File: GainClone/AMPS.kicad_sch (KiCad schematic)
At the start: 26 parts, among them U1 LM3886, U3 LM3886

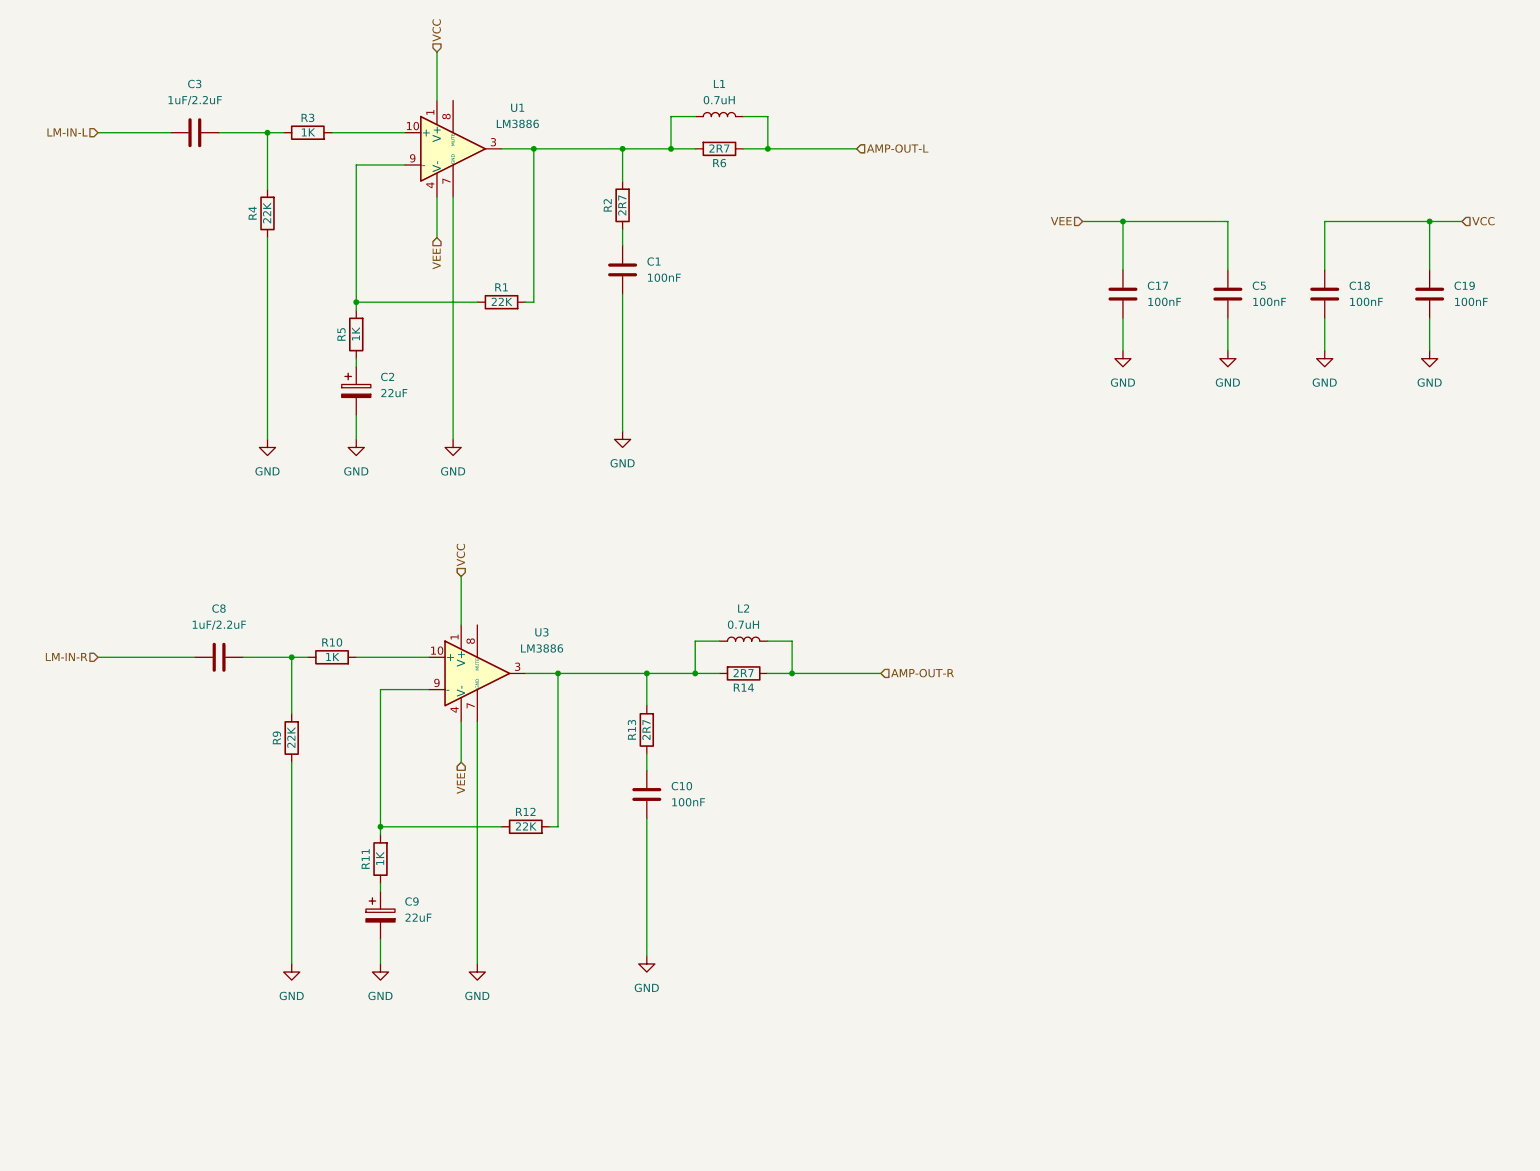
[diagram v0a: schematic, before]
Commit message: commit
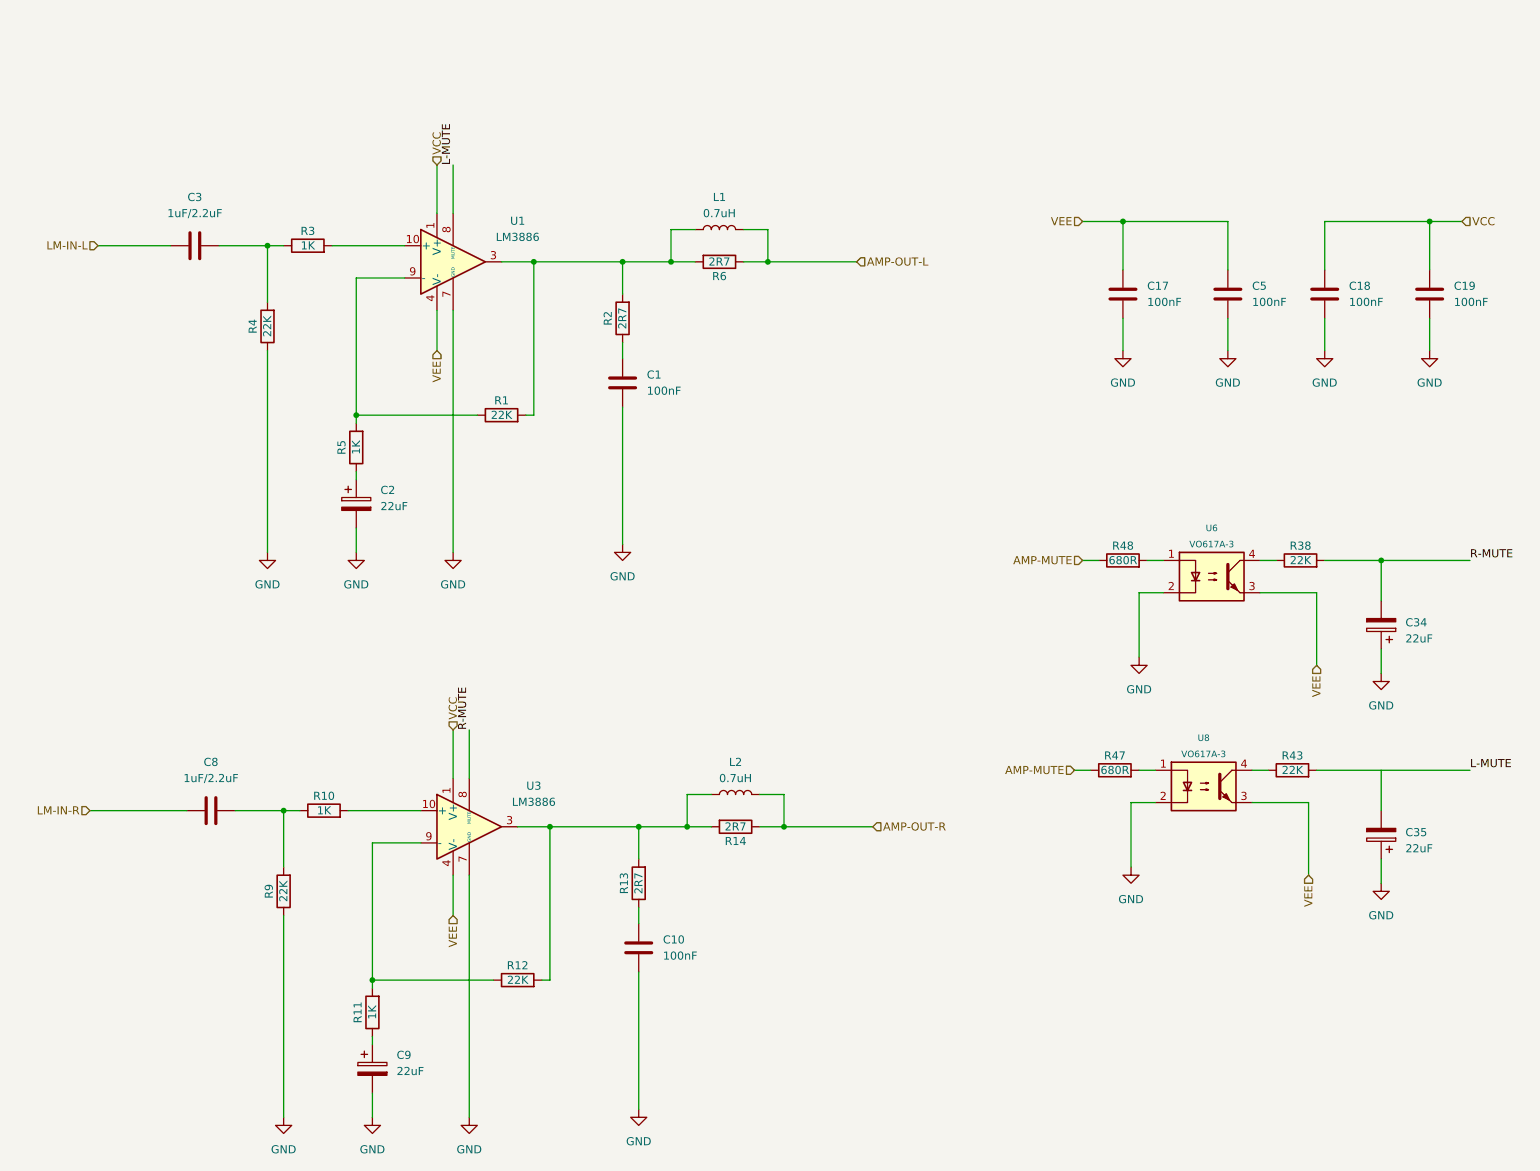
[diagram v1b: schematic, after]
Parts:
- added C34, C35: 22uF, Capacitor_THT:CP_Radial_D5.0mm_P2.50mm, symbol Device:C_Polarized
- added R38, R43: 22K, Resistor_SMD:R_0805_2012Metric_Pad1.20x1.40mm_HandSolder, symbol Device:R
- added R47, R48: 680R, Resistor_SMD:R_0805_2012Metric_Pad1.20x1.40mm_HandSolder, symbol Device:R
- added U6, U8: VO617A-3, Package_DIP:DIP-4_W7.62mm, symbol InputSwitch:VO617A_3
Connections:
- net GND: now also C34.1, C35.1, U6.2, U8.2
- net VEE: now also U6.3, U8.3
- net L-MUTE: now reaches U1.8 (MUTE)
- net L-MUTE: now also R43.2
- net R-MUTE: now reaches U3.8 (MUTE)
- net R-MUTE: now also C34.2, R38.2
- new net: R43.1, U8.4
- new net: R47.2, U8.1
- new net: R48.2, U6.1
- new net: R38.1, U6.4
- new net AMP-MUTE: R47.1, R48.1
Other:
- moved on the sheet: C1, C10, C2, C3, C8, C9, L1, L2, R1, R10, R11, R12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
